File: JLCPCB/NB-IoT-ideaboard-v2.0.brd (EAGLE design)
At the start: 93 x 65 mm, 111 parts, among them Q1 32.768kHz, Q3 9013, Q4 9013, Q5 9013, U1 STM32F103RBT6, U2 MCP73831T-2ACI/OT, U3 AP2112-3.3, U4 PAM2401, U5 MICROSIM, U6 BC92, U7 SIM-ST-MFF2, X1 8MHz

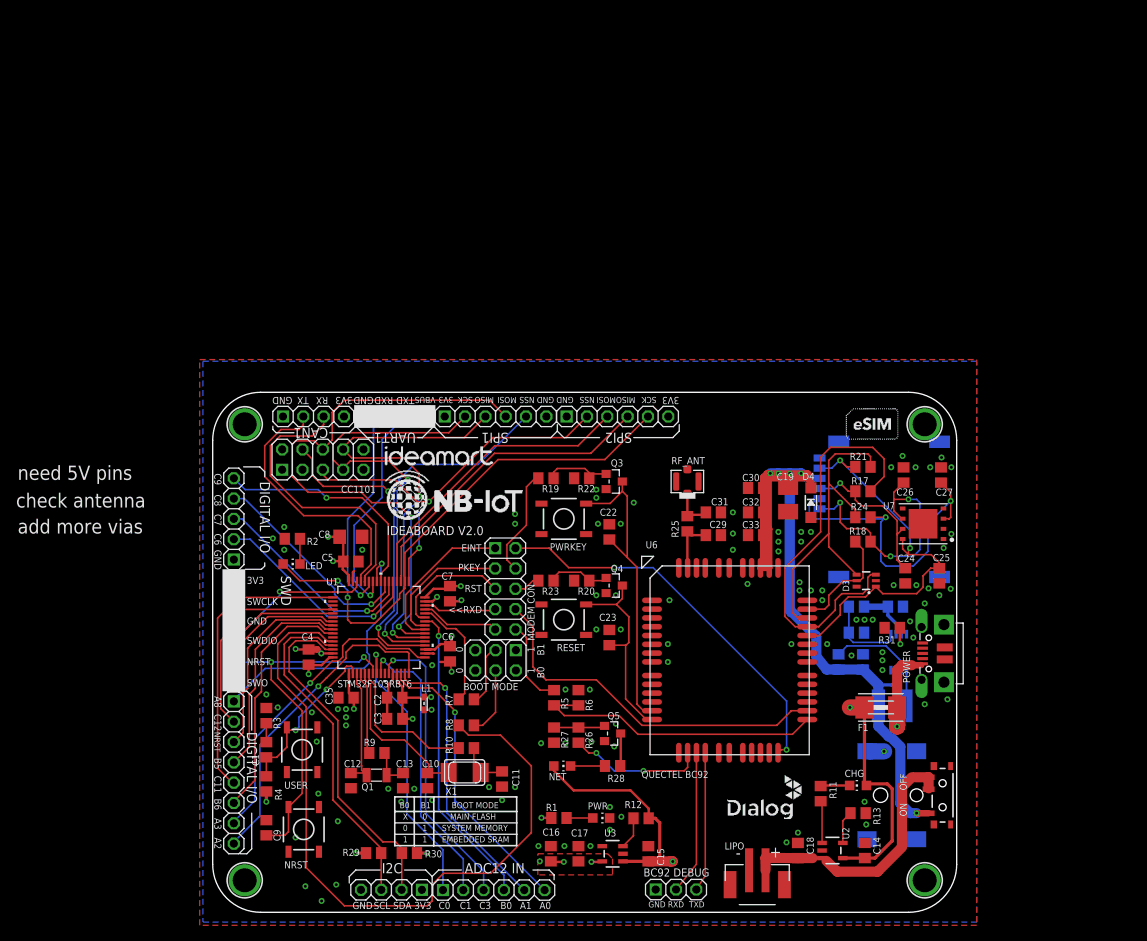
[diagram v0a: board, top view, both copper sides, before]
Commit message: JLCPCB layout antenna layout edits
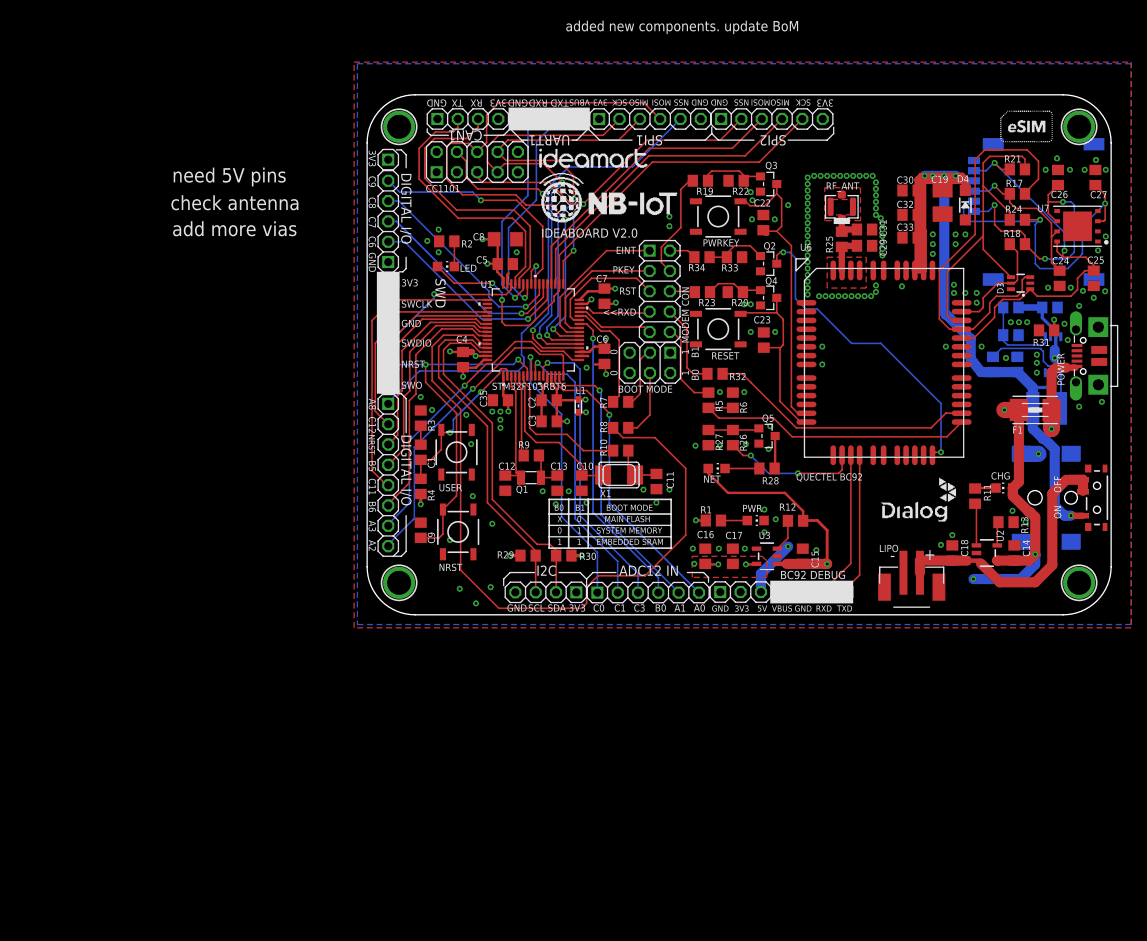
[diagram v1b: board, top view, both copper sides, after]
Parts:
- added JP3: (no value), pinhead-2:1X01-S
- added POWER-PINS: (no value), pinhead-2:1X04-S
- added Q2: 9013, discrete:SOT23
- added R32: 1k, rcl:R0805
- added R33: 47k, rcl:R0805
- added R34: 4k7, rcl:R0805
- moved C22 43.2 mm to (68.8, 86.2)
- moved S3 42.4 mm to (63.2, 87.0)
- moved C21 42.1 mm to (104.6, 75.6)
- moved R15 42.1 mm to (99.8, 75.6)
- moved BOOT 41.9 mm to (54.7, 68.7)
- moved C24 41.9 mm to (105.9, 79.2)
- moved C25 41.9 mm to (110.1, 79.2)
- moved CAN 41.9 mm to (31.9, 99.2)
- moved Q3 41.9 mm to (69.5, 91.0)
- moved R17 41.9 mm to (100.6, 89.8)
- moved R22 41.9 mm to (65.4, 91.4)
- moved SPI1 41.9 mm to (54.7, 99.2)
- moved SPI2 41.9 mm to (69.9, 99.2)
- moved U1 41.9 mm to (40.1, 72.8)
- moved U5 41.9 mm to (96.0, 95.2)
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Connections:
- new net N$17: MODEMCTL.8, R32.2
- new net N$23: Q2.1, R33.1, R34.1
- new net PSM_EINT: MODEMCTL.2, R34.2
- net +3V3: now also JP3.1, POWER-PINS.2
- net +5V: now also POWER-PINS.3
- net BC92_PSM_EINT: now also Q2.3; no longer MODEMCTL.2
- net BC92_TX: now also R32.1; no longer MODEMCTL.8
- net GND: now also POWER-PINS.1, Q2.2, R33.2
- net VBUS: now also POWER-PINS.4
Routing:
- net +5V: track 7.11 -> 62.8 mm, vias 0 -> 2
- net VBUS: track 105.7 -> 135.6 mm, vias 1 -> 3
- net BC92_TX: track 46.2 -> 33.4 mm
- net N$17: track 0.00 -> 10.8 mm
- net BC92_PSM_EINT: track 49.1 -> 39.8 mm
- net N$23: track 0.00 -> 7.79 mm
- net PSM_EINT: track 0.00 -> 3.40 mm
- net RF_ANT: track 7.08 -> 4.91 mm
- net V+: track 165.7 -> 167.6 mm
- net +4.1V: track 33.4 -> 35.1 mm
- net N$6: track 5.23 -> 3.60 mm
- net N$20: track 4.12 -> 2.97 mm
- net N$9: track 3.65 -> 2.63 mm
- net PA3: track 39.9 -> 39.0 mm
- net +3V3: track 44.1 -> 43.3 mm
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- added copper zone on layer 2, net N$13
- added copper zone on layer 15, net N$14
- added copper zone on layer 1, net N$15
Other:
- board text added: "5V"
- board text added: "added new components. update BoM"
